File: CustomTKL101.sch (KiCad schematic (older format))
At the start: 10 parts

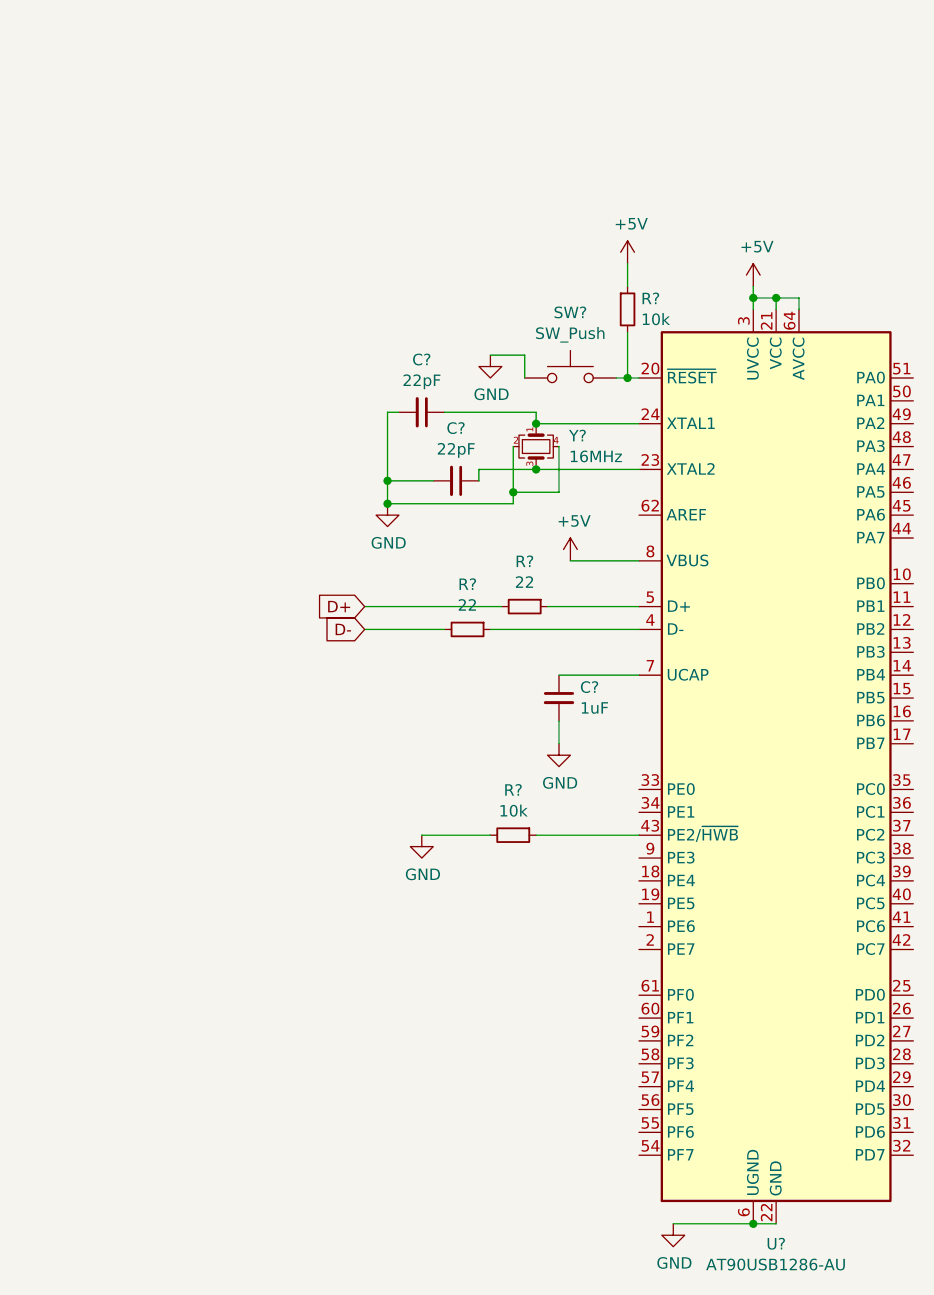
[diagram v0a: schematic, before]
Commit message: 15-02-2020
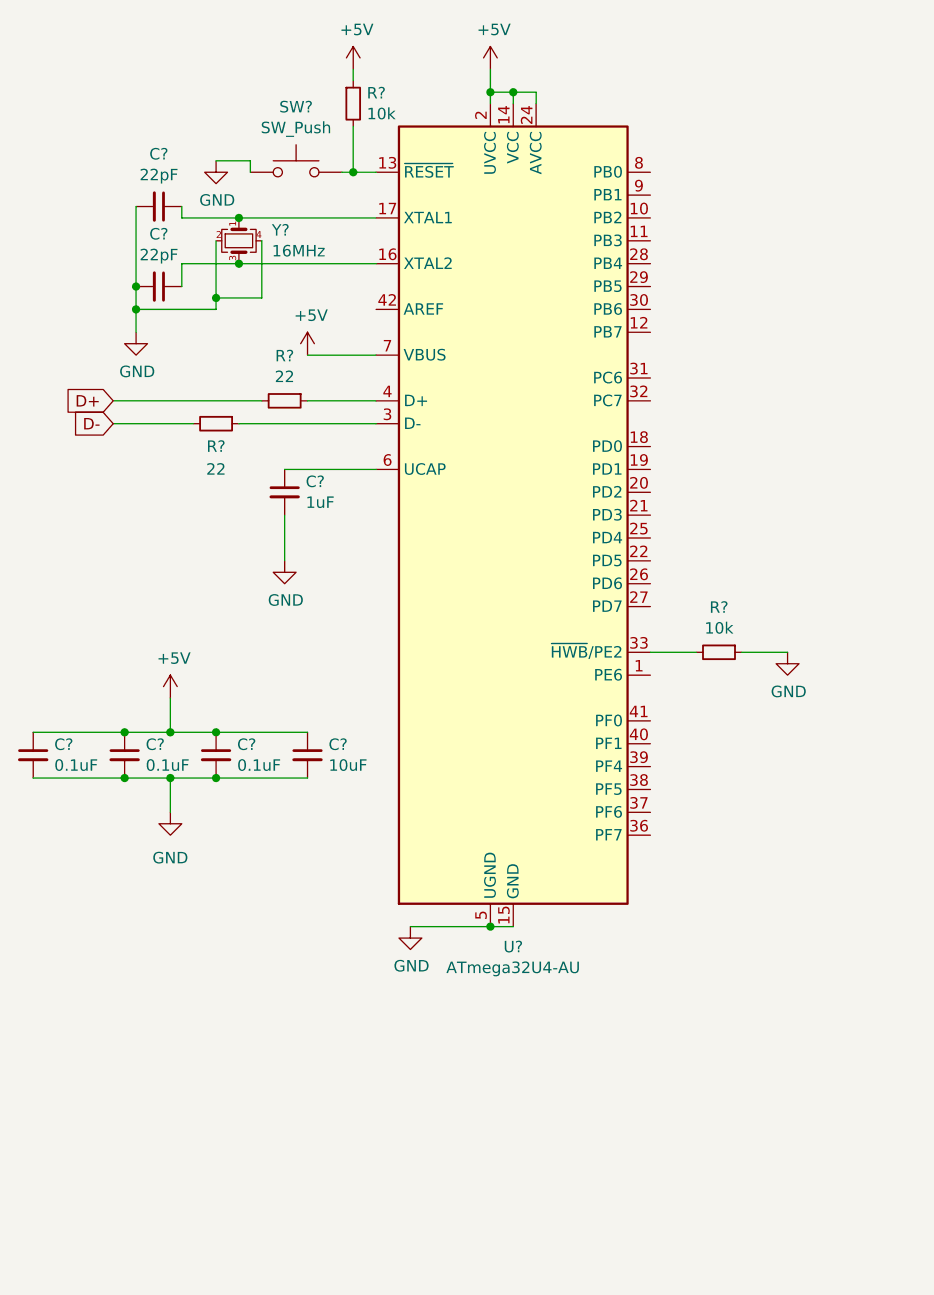
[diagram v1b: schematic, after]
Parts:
- removed C?: 1uF, symbol Device:C_Small
- removed C? (x2): 22pF, symbol Device:C_Small
- removed R? (x2): 10k, symbol Device:R_Small
- removed R? (x2): 22, symbol Device:R_Small
- removed SW?: SW_Push, symbol Switch:SW_Push
- removed U?: AT90USB1286-AU, Package_QFP:TQFP-64_14x14mm_P0.8mm, symbol MCU_Microchip_AVR:AT90USB1286-AU
- removed Y?: 16MHz, symbol Device:Crystal_GND24_Small
- added C?: 1uF, symbol Device:C_Small
- added C?: 10uF, symbol Device:C_Small
- added C? (x3): 0.1uF, symbol Device:C_Small
- added C? (x2): 22pF, symbol Device:C_Small
- added R? (x2): 10k, symbol Device:R_Small
- added R? (x2): 22, symbol Device:R_Small
- added SW?: SW_Push, symbol Switch:SW_Push
- added U?: ATmega32U4-AU, Package_QFP:TQFP-44_10x10mm_P0.8mm, symbol MCU_Microchip_ATmega:ATmega32U4-AU
- added Y?: 16MHz, symbol Device:Crystal_GND24_Small
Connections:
- net +5V: now also C?.1, C?.1, C?.1, C?.1, R?.1, U?.14 (VCC), U?.2 (UVCC), U?.24 (AVCC), U?.34 (VCC), U?.44 (AVCC), U?.7 (VBUS)
- net D+: now also R?.2
- net D-: now also R?.2
- net GND: now also C?.2, C?.2, C?.2, C?.2, C?.2, C?.2, C?.2, R?.1, SW?.1, U?.15 (GND), U?.23 (GND), U?.35 (GND), U?.43 (GND), U?.5 (UGND), Y?.2, Y?.4
- new net: R?.2, SW?.2, U?.13 (~RESET)
- new net: C?.1, U?.16 (XTAL2), Y?.3
- new net: C?.1, U?.17 (XTAL1), Y?.1
- new net: R?.1, U?.3 (D-)
- new net: R?.2, U?.33 (~HWB~/PE2)
- new net: R?.1, U?.4 (D+)
- new net: C?.1, U?.6 (UCAP)
